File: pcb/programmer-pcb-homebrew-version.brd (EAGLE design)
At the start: 17 x 56.9 mm, 10 parts, among them IC1 MEGA8-AI, IC2 FT232RL, Q1 16 MHz

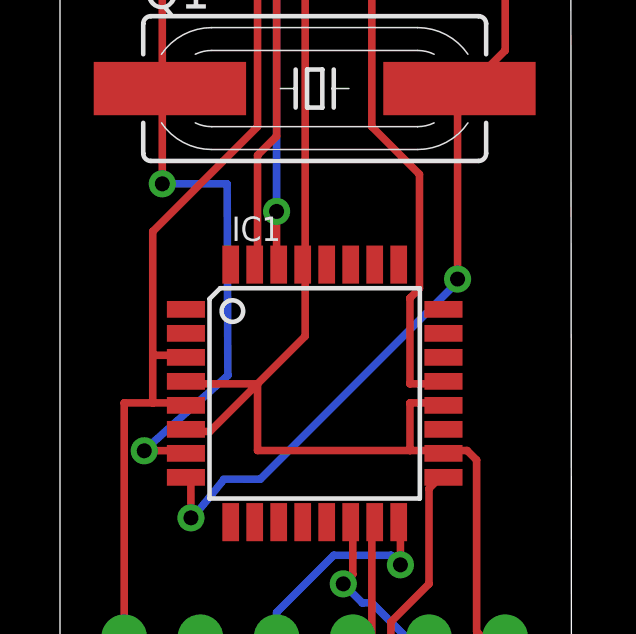
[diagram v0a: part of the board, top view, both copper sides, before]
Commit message: Minor changes
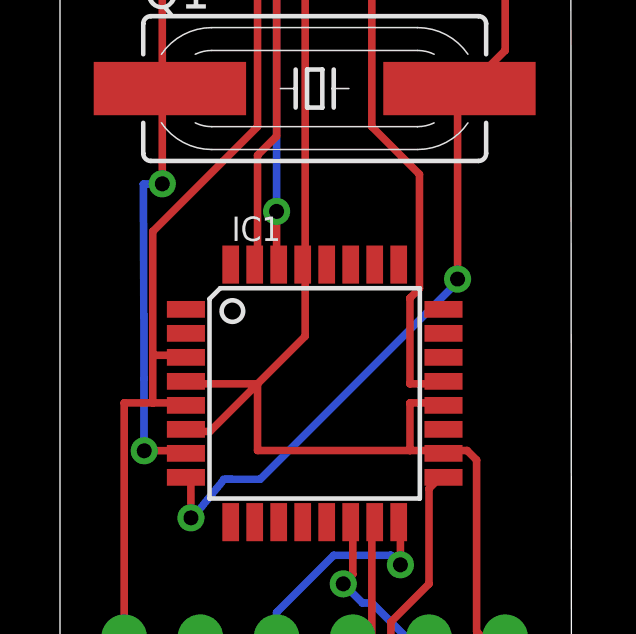
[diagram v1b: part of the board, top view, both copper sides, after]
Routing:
- net N$4: track 12.2 -> 10.7 mm
- net S$28: track 10.2 -> 8.90 mm
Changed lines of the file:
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@@
 <contactref element="C2" pad="1"/>
 <contactref element="Q1" pad="1"/>
-<wire x1="5.08" y1="19.685" x2="7.240178125" y2="19.685" width="0.254" layer="16"/>
+<wire x1="5.08" y1="19.685" x2="4.44785625" y2="19.67254375" width="0.254" layer="16"/>
 <wire x1="5.08" y1="22.86" x2="5.08" y2="19.685" width="0.254" layer="1"/>
 <wire x1="5.08" y1="22.86" x2="5.08" y2="29.21" width="0.254" layer="1"/>
@@
 </signal>
 <signal name="S$28">
-<wire x1="7.241165625" y1="19.67993125" x2="7.265975" y2="13.297084375" width="0.254" layer="16"/>
-<wire x1="7.265975" y1="13.297084375" x2="4.468321875" y2="10.791303125" width="0.254" layer="16"/>
+<wire x1="4.44874375" y1="19.67405" x2="4.47365" y2="13.184984375" width="0.254" layer="16"/>
+<wire x1="4.47365" y1="13.184984375" x2="4.468321875" y2="10.791303125" width="0.254" layer="16"/>
 <wire x1="4.468321875" y1="10.791303125" x2="4.47433125" y2="10.780275" width="0.254" layer="16"/>
 </signal>
